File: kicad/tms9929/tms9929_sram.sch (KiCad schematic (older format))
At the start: 64 parts, among them P1 CONN_01X03, P4 Power, Q1 BC550, Q10 BC550, Q2 BC550, Q3 BC550, Q4 BC550, Q5 BC550, Q6 BC550, Q7 BC550, Q8 BC550, Q9 BC550, U1 TMS9929A, U10 7400, U2 74HCT04, U3 74HCT574, U4 74HCT574, U5 74HCT574, U6 HM62256BLFP-5SLT

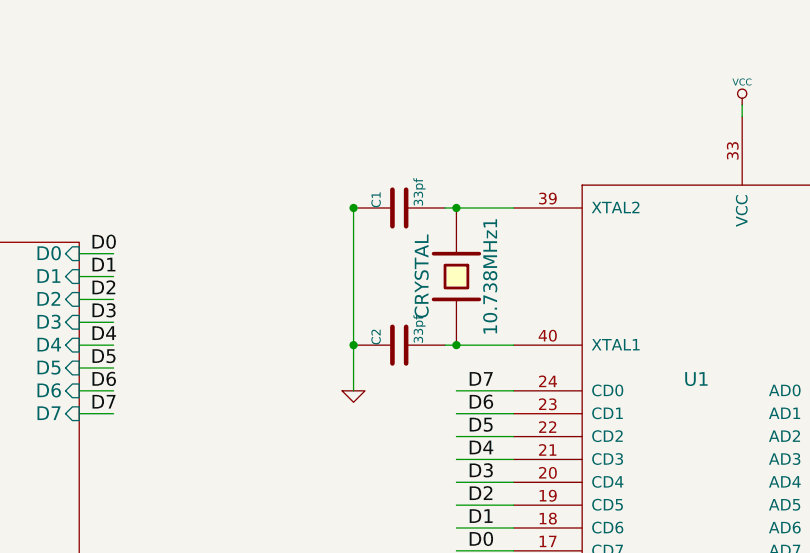
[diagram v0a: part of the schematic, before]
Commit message: +update rev.1.1
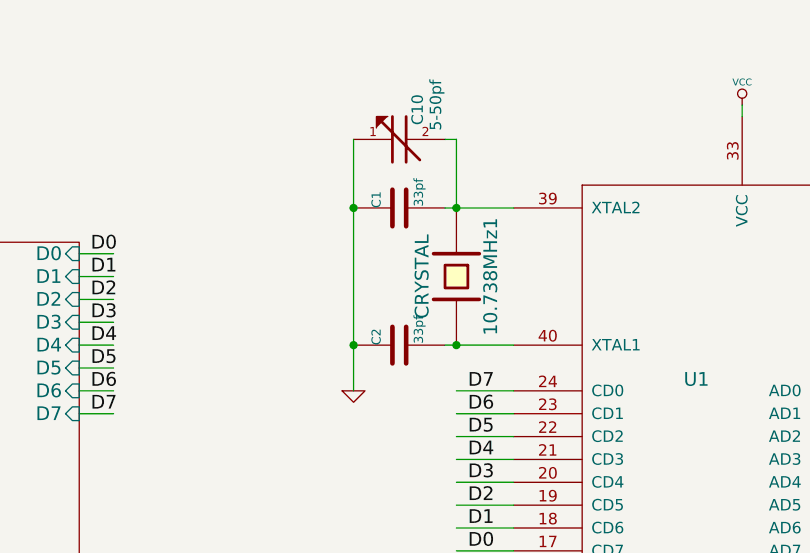
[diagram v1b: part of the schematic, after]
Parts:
- added C10: 5-50pf, symbol CTRIM
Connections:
- wire segments 280 -> 282
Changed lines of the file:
@@
 LIBS:valves
 LIBS:tms99xx
-LIBS:tms9929_sram_snd-cache
 EELAYER 24 0
 EELAYER END
@@
 	1850 7450 2050 7450
 Wire Wire Line
-	3650 1350 3650 2150
+	3650 1050 3650 2150
 Wire Wire Line
 	13700 3550 13700 3650
@@
 Connection ~ 3400 6900
 Connection ~ 3650 6900
+$Comp
+L CTRIM C10
+U 1 1 5526BE0E
+P 3850 1050
+F 0 "C10" H 3980 970 50  0000 C CNN
+F 1 "5-50pf" H 4000 890 50  0000 C CNN
+F 2 "" H 3850 1050 60  0000 C CNN
+F 3 "" H 3850 1050 60  0000 C CNN
+	1    3850 1050
+	0    -1   -1   0
+$EndComp
+Wire Wire Line
+	4050 1050 4100 1050
+Wire Wire Line
+	4100 1050 4100 1350
 $EndSCHEMATC
